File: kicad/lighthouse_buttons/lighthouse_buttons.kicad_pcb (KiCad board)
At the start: 2 copper layers, 128 x 8 mm, 8 parts, among them J1 Conn_01x06_Pin

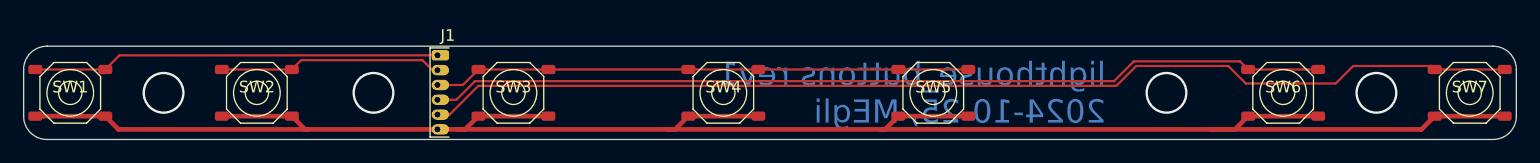
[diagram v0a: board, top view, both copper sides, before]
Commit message: hardware for lighthouse display rev1 and button rev1 done
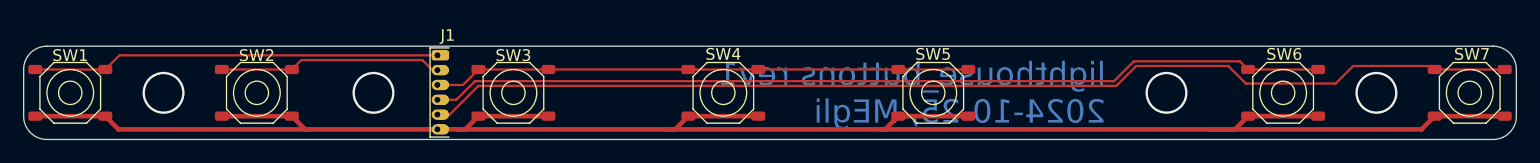
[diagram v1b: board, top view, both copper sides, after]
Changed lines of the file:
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@@
 		(at 204 94.4)
 		(property "Reference" "SW7"
-			(at 0 -0.5 0)
+			(at 0.2 -3.3 0)
 			(unlocked yes)
 			(layer "F.SilkS")
@@
 		(at 158 94.4)
 		(property "Reference" "SW5"
-			(at 0 -0.5 0)
+			(at 0 -3.3 0)
 			(unlocked yes)
 			(layer "F.SilkS")
@@
 		(at 100 94.4)
 		(property "Reference" "SW2"
-			(at 0 -0.5 0)
+			(at 0 -3.2 0)
 			(unlocked yes)
 			(layer "F.SilkS")
@@
 		(at 140 94.4)
 		(property "Reference" "SW4"
-			(at 0 -0.5 0)
+			(at 0 -3.3 0)
 			(unlocked yes)
 			(layer "F.SilkS")
@@
 		(at 84 94.4)
 		(property "Reference" "SW1"
-			(at 0 -0.5 0)
+			(at 0 -3.2 0)
 			(unlocked yes)
 			(layer "F.SilkS")
@@
 		(at 122 94.4)
 		(property "Reference" "SW3"
-			(at 0 -0.5 0)
+			(at 0 -3.2 0)
 			(unlocked yes)
 			(layer "F.SilkS")
@@
 		(at 188 94.4)
 		(property "Reference" "SW6"
-			(at 0 -0.5 0)
+			(at 0.1 -3.3 0)
 			(unlocked yes)
 			(layer "F.SilkS")
@@
 		)
 	)
+	(dimension
+		(type aligned)
+		(layer "Eco1.User")
+		(pts
+			(xy 82.2 90.4) (xy 82.2 98.4)
+		)
+		(height 4.2)
+		(gr_text "8.0 mm"
+			(at 76.85 94.4 90)
+			(layer "Eco1.User")
+			(effects
+				(font
+					(size 1 1)
+					(thickness 0.15)
+				)
+			)
+		)
+		(format
+			(prefix "")
+			(suffix "")
+			(units 3)
+			(units_format 1)
+			(precision 1)
+		)
+		(style
+			(thickness 0.1)
+			(arrow_length 1.27)
+			(text_position_mode 0)
+			(extension_height 0.58642)
+			(extension_offset 0.5) keep_text_aligned)
+	)
+	(dimension
+		(type aligned)
+		(layer "Eco1.User")
+		(pts
+			(xy 80 92.4) (xy 208 92.4)
+		)
+		(height -4.4)
+		(gr_text "128.0 mm"
+			(at 144 86.85 0)
+			(layer "Eco1.User")
+			(effects
+				(font
+					(size 1 1)
+					(thickness 0.15)
+				)
+			)
+		)
+		(format
+			(prefix "")
+			(suffix "")
+			(units 3)
+			(units_format 1)
+			(precision 1)
+		)
+		(style
+			(thickness 0.1)
+			(arrow_length 1.27)
+			(text_position_mode 0)
+			(extension_height 0.58642)
+			(extension_offset 0.5) keep_text_aligned)
+	)
 	(via
